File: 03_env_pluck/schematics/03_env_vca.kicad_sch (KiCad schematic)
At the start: 45 parts, among them J1 gate in 1, J2 signal in, J3 Eurorack, J4 Signal out, J5 Env out 1, Q1 BC847, Q2 BC847, SW1 Pluck / AD 1, U1 TL072, U2 LM358

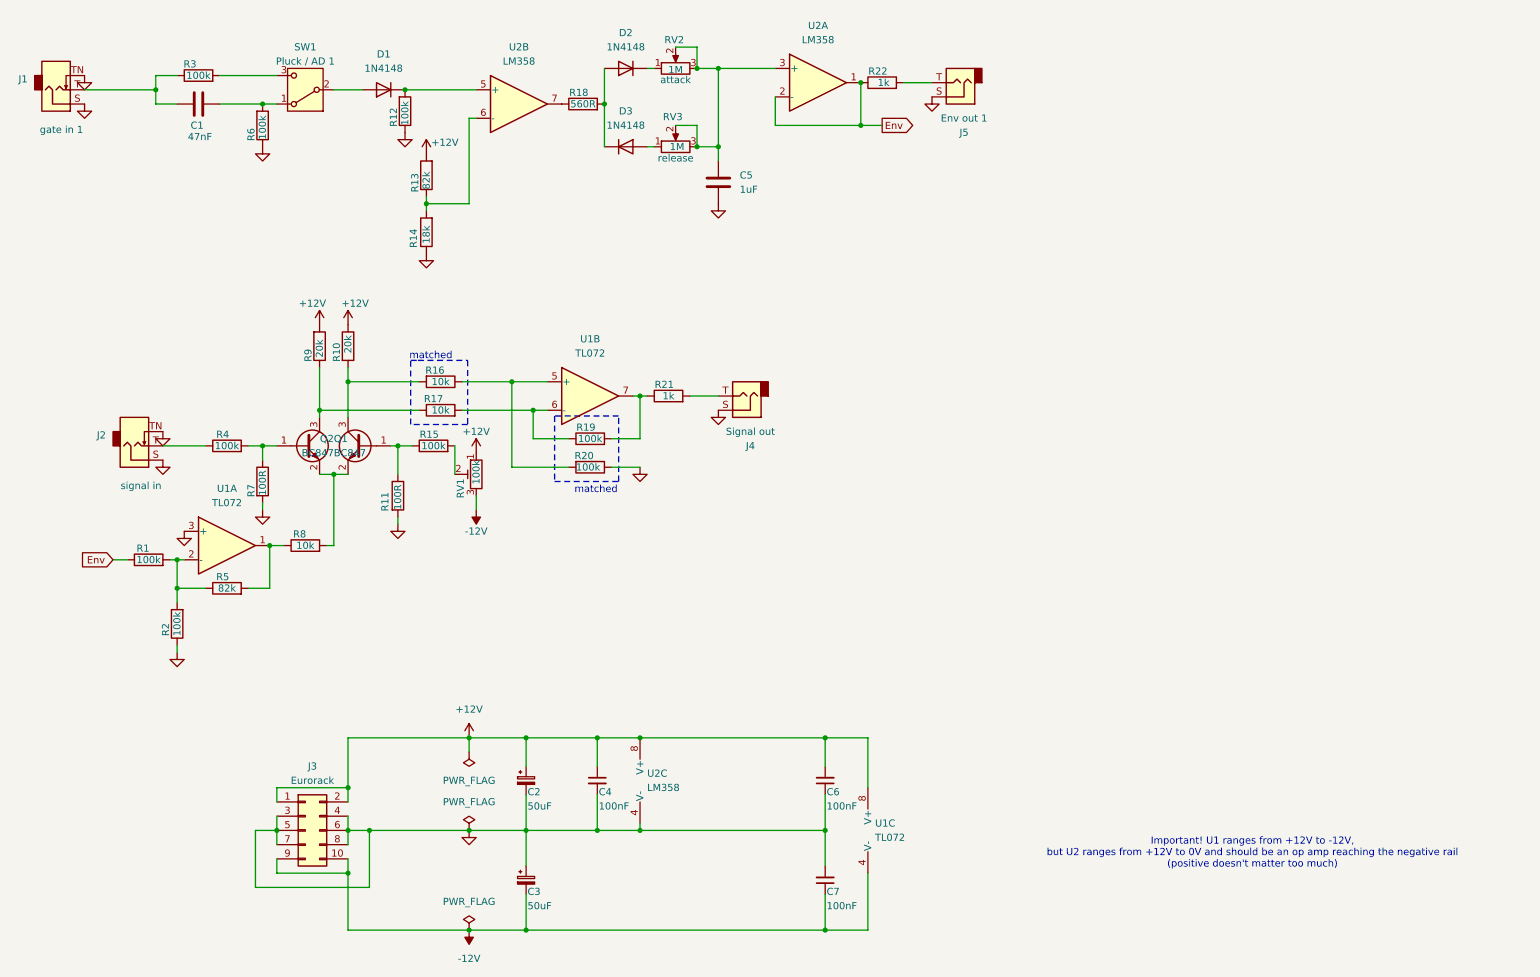
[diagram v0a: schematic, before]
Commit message: cleanup
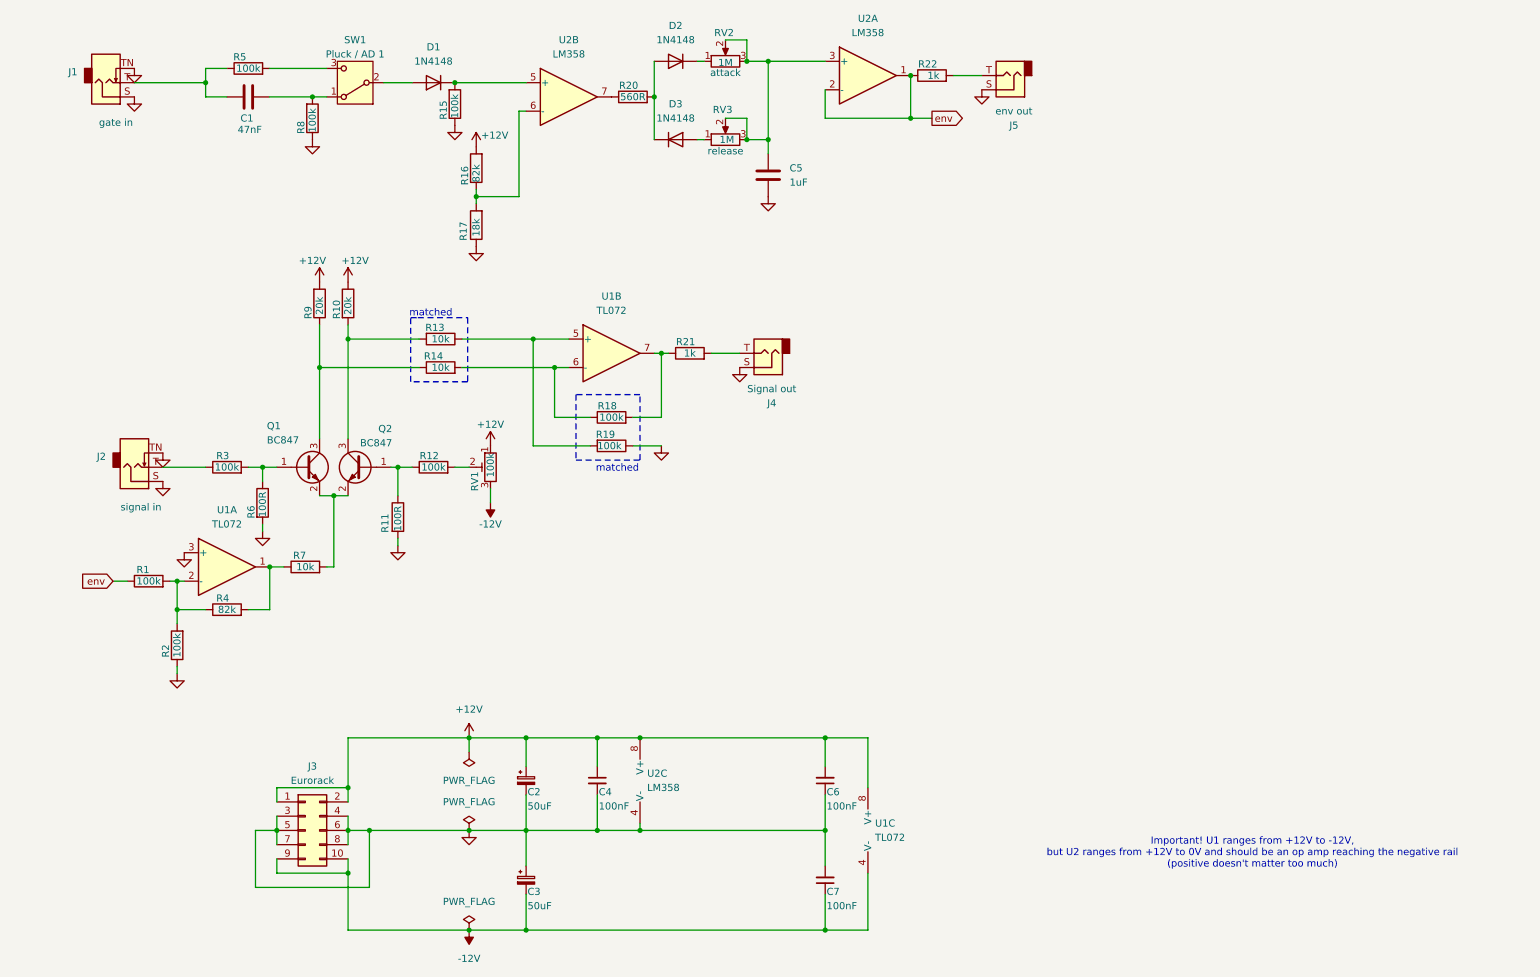
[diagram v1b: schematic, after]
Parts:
- J1: value gate in 1 -> gate in
- J5: value Env out 1 -> env out
- renumbered R15 to R12, R16 to R13, R17 to R14, R12 to R15, R13 to R16, R14 to R17, R19 to R18, R20 to R19, R18 to R20, R4 to R3, R5 to R4, R3 to R5, R7 to R6, R8 to R7, R6 to R8
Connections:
- net Env renamed env
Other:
- moved on the sheet: C1, C5, D1, D2, D3, J1, J2, J4, J5, Q1, Q2, R1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
